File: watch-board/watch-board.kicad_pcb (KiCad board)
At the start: 2 copper layers, 34 x 34 mm, 64 parts, among them J1 Conn_PAD, J2 Conn_PAD, J3 Conn_PAD, J4 Conn_PAD, J5 Conn_PAD, Q1 Phototransistor_ALS-PT19-315C, Q2 Phototransistor_ALS-PT19-315C, Q3 Transistor_MMBT3904-TP, U1 Display-Driver_PCA8561ANH, U2 Regulator_BQ25504, U3 Regulator_LTC3531-3, U4 MCU_STM32L051K8Ux

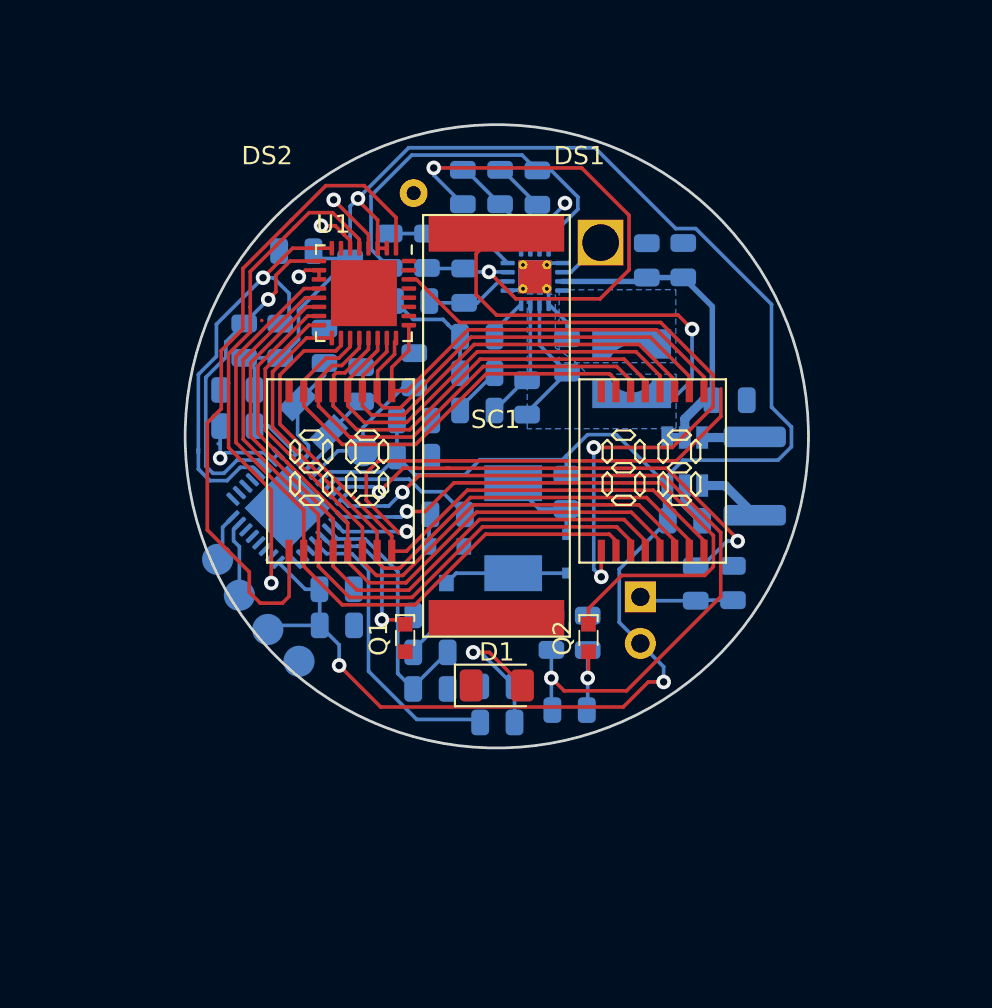
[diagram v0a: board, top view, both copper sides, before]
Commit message: finished wiring
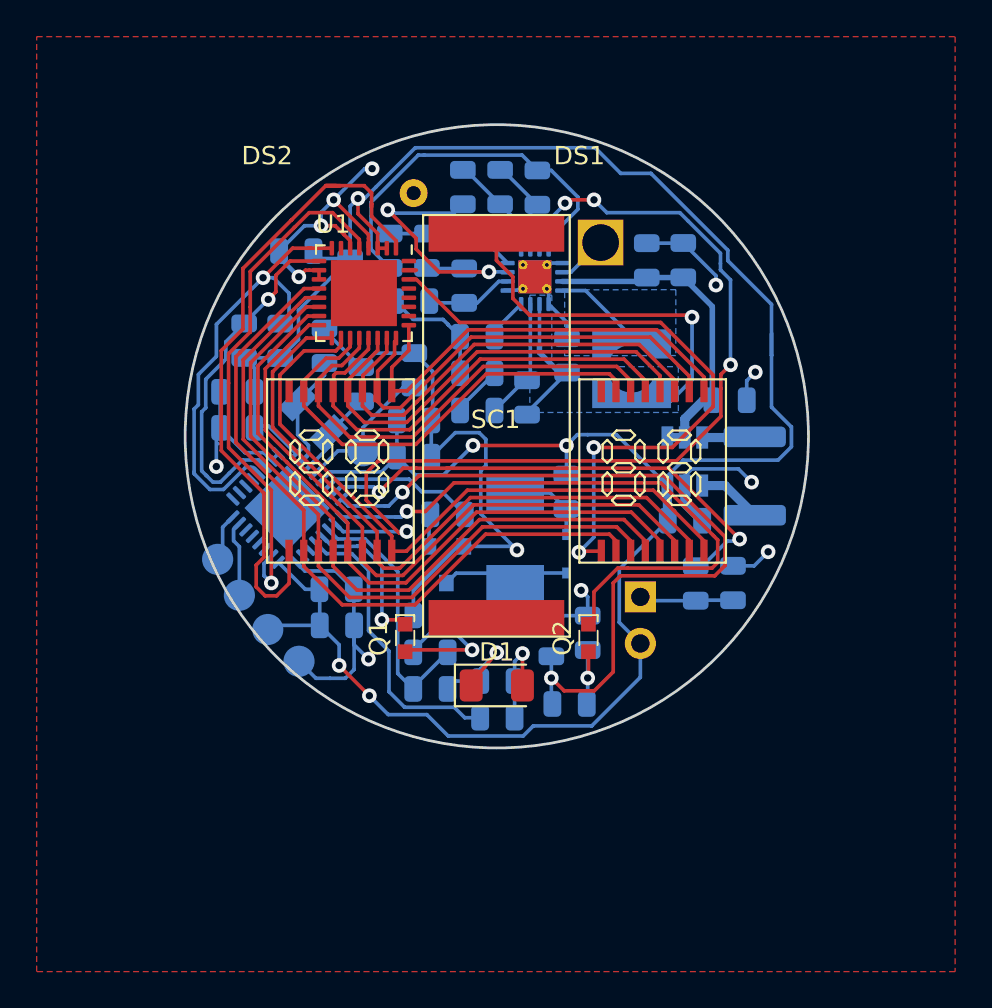
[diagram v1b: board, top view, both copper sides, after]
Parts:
- moved BZ1 0.54 mm to (141.0, 105.5)
- moved C19 0.35 mm to (143.0, 111.1)
- moved R21 0.34 mm to (144.0, 114.6)
- moved R22 0.29 mm to (140.0, 113.3)
- moved R15 0.26 mm to (140.0, 115.3)
- moved C12 0.10 mm to (125.8, 97.6)
- moved C13 0.10 mm to (125.8, 99.5)
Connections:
- DS1 pad 2: GND -> /1G
- DS2 pad 2: GND -> /1G
- U1 pad 12: GND -> /1G
- U1 pad 31: /COM2 -> Net-(U1-Pad31)
- U1 pad 32: /COM1 -> Net-(U1-Pad32)
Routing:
- net GND: track 91.8 -> 135.9 mm, vias 4 -> 13
- net /1G: track 0.00 -> 39.2 mm
- net /VBAT_OK: track 33.8 -> 51.5 mm, vias 2 -> 4
- net Net-(R1-Pad1): track 30.4 -> 15.8 mm
- net Net-(Q1-Pad2): track 2.80 -> 9.17 mm, vias 0 -> 1
- net Net-(L1-Pad2): track 0.00 -> 4.83 mm
- net Net-(D1-Pad2): track 8.44 -> 5.42 mm
- net VDD: track 136.3 -> 138.3 mm, vias 3 -> 5
- net /LIGHT_R: track 41.3 -> 43.1 mm
- net /RESET: track 27.0 -> 28.8 mm
- net Net-(C2-Pad1): track 30.7 -> 29.1 mm
- net /COM1: track 36.5 -> 35.3 mm
- net /SCL: track 24.2 -> 25.4 mm
- net /SDA: track 18.5 -> 19.6 mm
- net /VLIGHT_R: track 32.8 -> 33.3 mm
- added copper zone on F.Cu, net GND
